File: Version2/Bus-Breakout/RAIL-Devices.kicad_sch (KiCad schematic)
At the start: 32 parts, among them J2 Conn_01x30_Pin, J5 Conn_02x30_Odd_Even, P1 Jumper4x1, P10 Jumper4x1, P11 Jumper4x1, P12 Jumper4x1, P13 Jumper4x1, P14 Jumper4x1, P15 Jumper4x1, P16 Jumper4x1, P17 Jumper4x1, P18 Jumper4x1, P19 Jumper4x1, P2 Jumper4x1, P20 Jumper4x1, P21 Jumper4x1, P22 Jumper4x1, P23 Jumper4x1, P24 Jumper4x1, P25 Jumper4x1, P26 Jumper4x1, P27 Jumper4x1, P28 Jumper4x1, P29 Jumper4x1, P3 Jumper4x1, P30 Jumper4x1, P4 Jumper4x1, P5 Jumper4x1, P6 Jumper4x1, P7 Jumper4x1, P8 Jumper4x1, P9 Jumper4x1

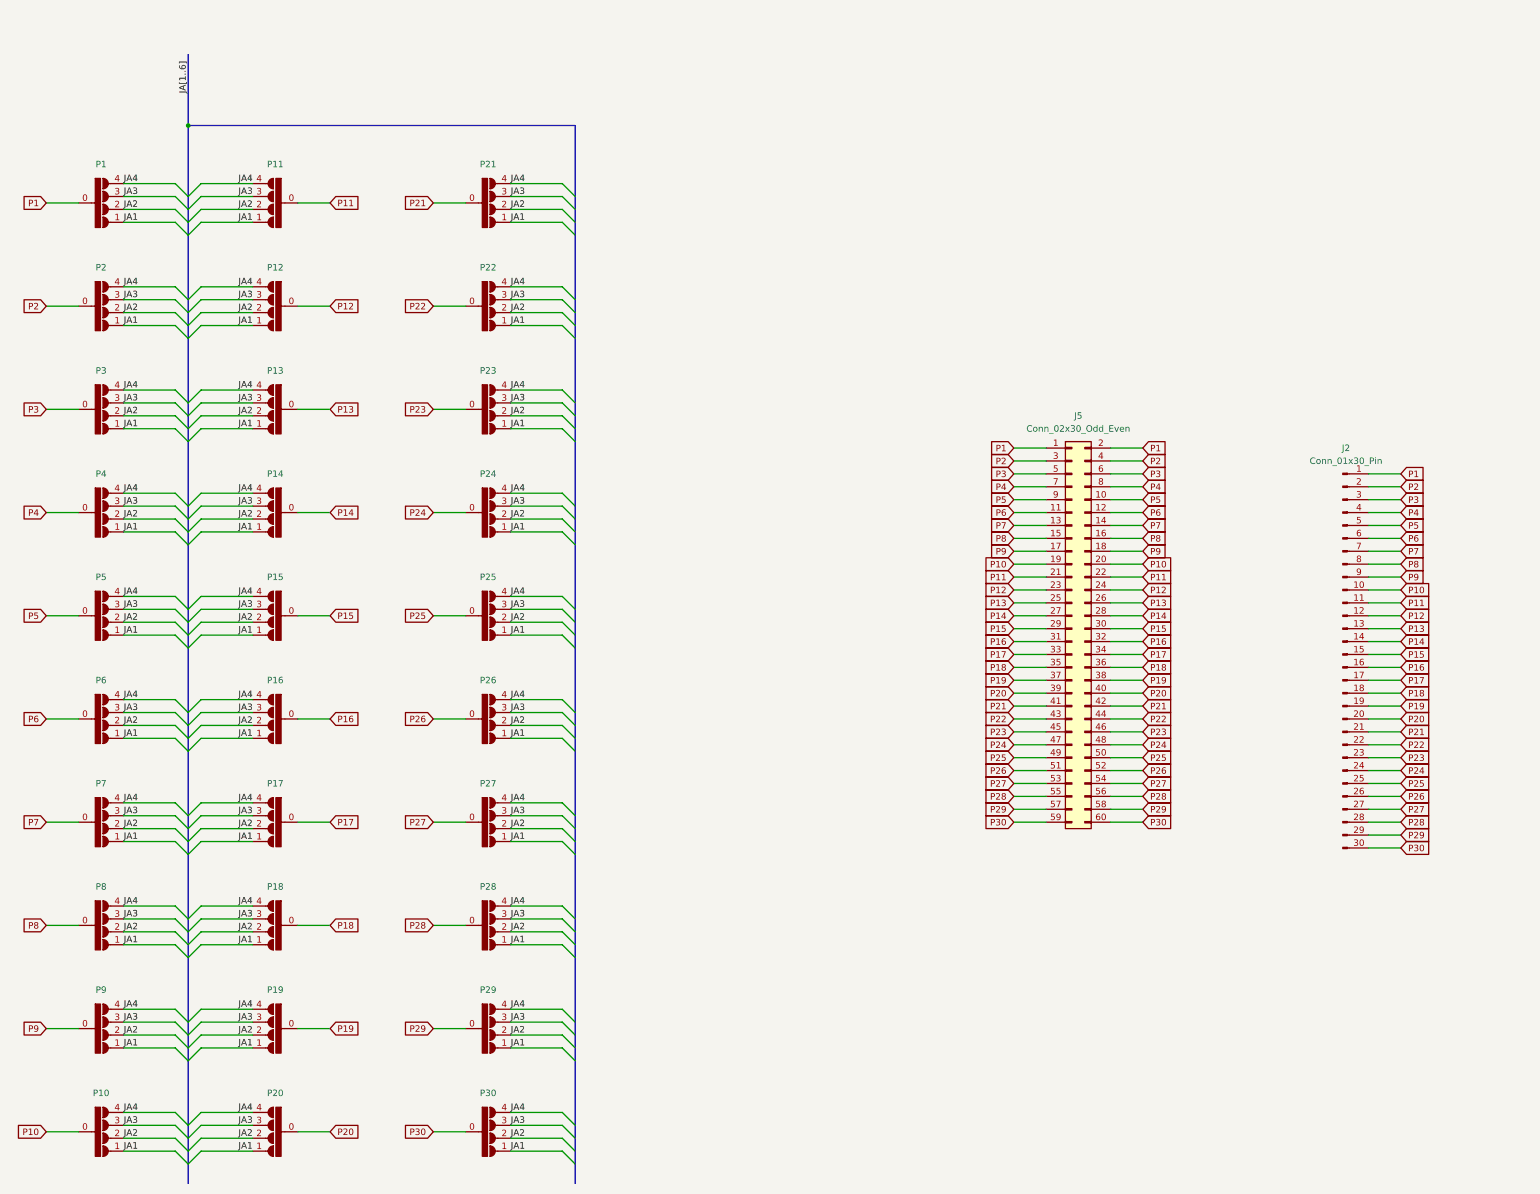
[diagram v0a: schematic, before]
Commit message: updates.
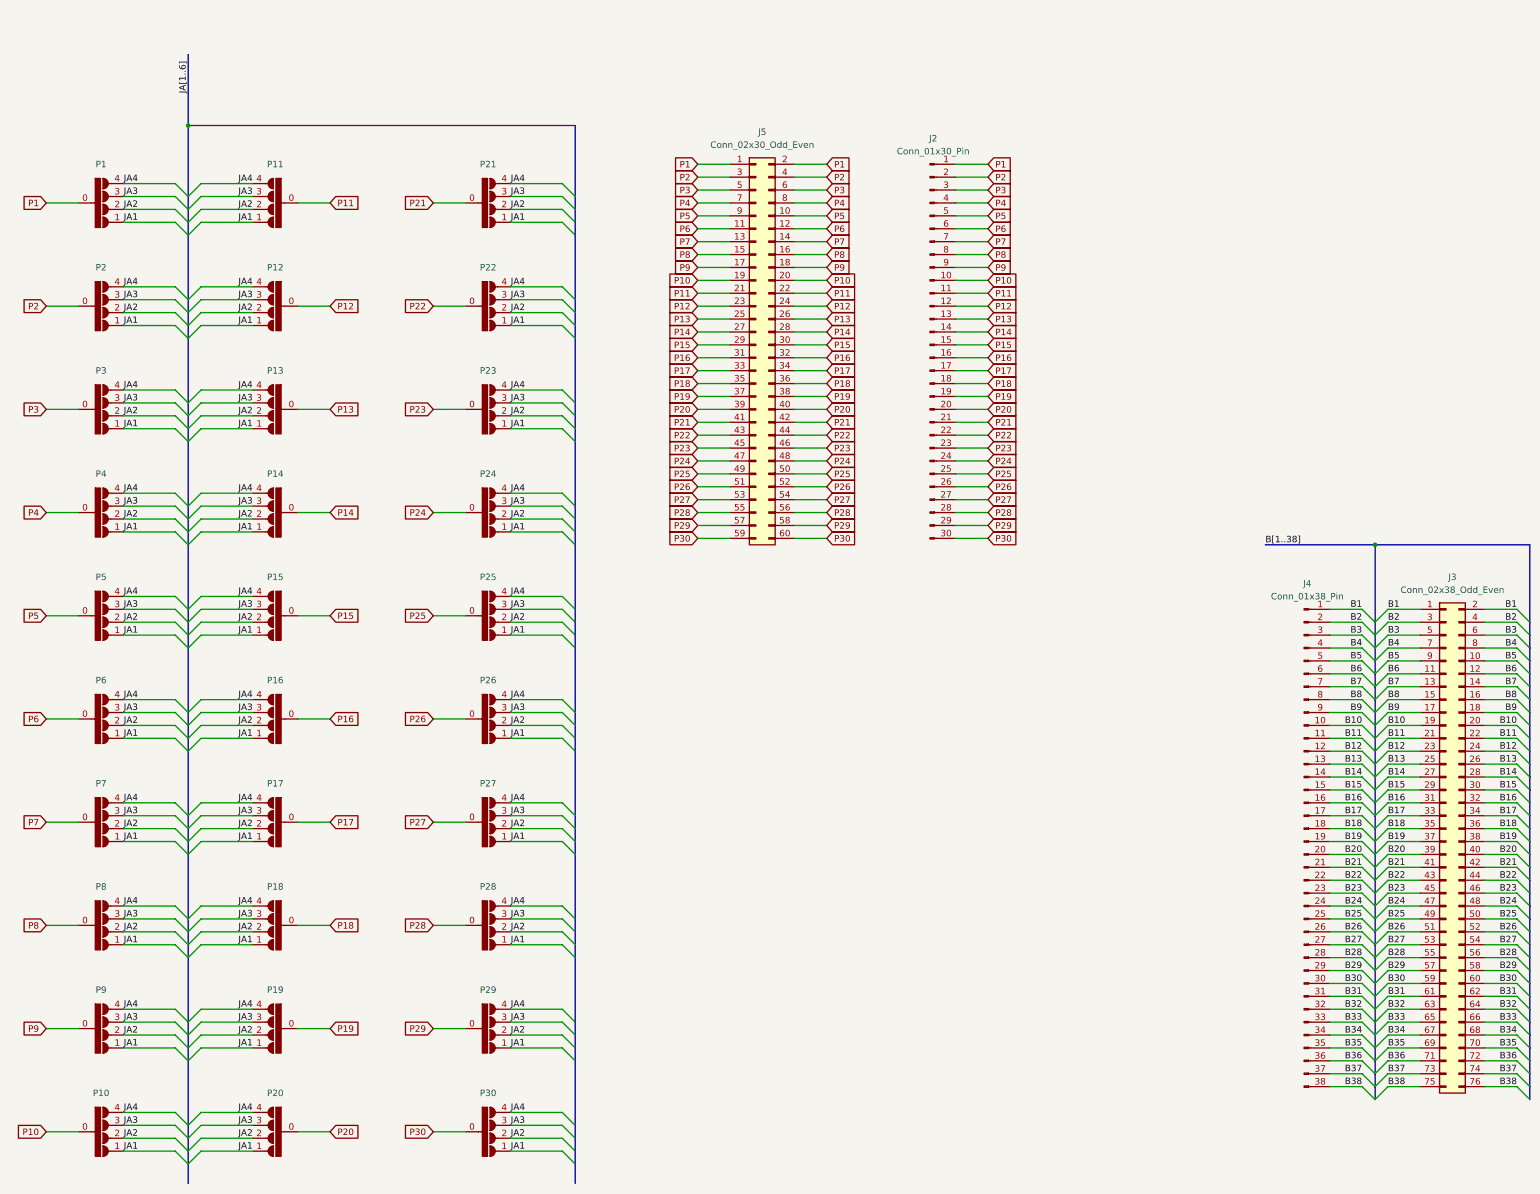
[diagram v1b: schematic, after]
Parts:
- added J3: Conn_02x38_Odd_Even, Connector_PinSocket_2.54mm:PinSocket_2x38_P2.54mm_Vertical, symbol Connector_Generic:Conn_02x38_Odd_Even
- added J4: Conn_01x38_Pin, Connector_PinSocket_2.54mm:PinSocket_1x38_P2.54mm_Vertical, symbol Connector:Conn_01x38_Pin
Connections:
- new net B1: J3.1 (Pin_1), J3.2 (Pin_2), J4.1 (Pin_1)
- new net B10: J3.19 (Pin_19), J3.20 (Pin_20), J4.10 (Pin_10)
- new net B11: J3.21 (Pin_21), J3.22 (Pin_22), J4.11 (Pin_11)
- new net B12: J3.23 (Pin_23), J3.24 (Pin_24), J4.12 (Pin_12)
- new net B13: J3.25 (Pin_25), J3.26 (Pin_26), J4.13 (Pin_13)
- new net B14: J3.27 (Pin_27), J3.28 (Pin_28), J4.14 (Pin_14)
- new net B15: J3.29 (Pin_29), J3.30 (Pin_30), J4.15 (Pin_15)
- new net B16: J3.31 (Pin_31), J3.32 (Pin_32), J4.16 (Pin_16)
- new net B17: J3.33 (Pin_33), J3.34 (Pin_34), J4.17 (Pin_17)
- new net B18: J3.35 (Pin_35), J3.36 (Pin_36), J4.18 (Pin_18)
- new net B19: J3.37 (Pin_37), J3.38 (Pin_38), J4.19 (Pin_19)
- new net B2: J3.3 (Pin_3), J3.4 (Pin_4), J4.2 (Pin_2)
- new net B20: J3.39 (Pin_39), J3.40 (Pin_40), J4.20 (Pin_20)
- new net B21: J3.41 (Pin_41), J3.42 (Pin_42), J4.21 (Pin_21)
- new net B22: J3.43 (Pin_43), J3.44 (Pin_44), J4.22 (Pin_22)
- new net B23: J3.45 (Pin_45), J3.46 (Pin_46), J4.23 (Pin_23)
- new net B24: J3.47 (Pin_47), J3.48 (Pin_48), J4.24 (Pin_24)
- new net B25: J3.49 (Pin_49), J3.50 (Pin_50), J4.25 (Pin_25)
- new net B26: J3.51 (Pin_51), J3.52 (Pin_52), J4.26 (Pin_26)
- new net B27: J3.53 (Pin_53), J3.54 (Pin_54), J4.27 (Pin_27)
- new net B28: J3.55 (Pin_55), J3.56 (Pin_56), J4.28 (Pin_28)
- new net B29: J3.57 (Pin_57), J3.58 (Pin_58), J4.29 (Pin_29)
- new net B3: J3.5 (Pin_5), J3.6 (Pin_6), J4.3 (Pin_3)
- new net B30: J3.59 (Pin_59), J3.60 (Pin_60), J4.30 (Pin_30)
- new net B31: J3.61 (Pin_61), J3.62 (Pin_62), J4.31 (Pin_31)
- new net B32: J3.63 (Pin_63), J3.64 (Pin_64), J4.32 (Pin_32)
- new net B33: J3.65 (Pin_65), J3.66 (Pin_66), J4.33 (Pin_33)
- new net B34: J3.67 (Pin_67), J3.68 (Pin_68), J4.34 (Pin_34)
- new net B35: J3.69 (Pin_69), J3.70 (Pin_70), J4.35 (Pin_35)
- new net B36: J3.71 (Pin_71), J3.72 (Pin_72), J4.36 (Pin_36)
- new net B37: J3.73 (Pin_73), J3.74 (Pin_74), J4.37 (Pin_37)
- new net B38: J3.75 (Pin_75), J3.76 (Pin_76), J4.38 (Pin_38)
- new net B4: J3.7 (Pin_7), J3.8 (Pin_8), J4.4 (Pin_4)
- new net B5: J3.10 (Pin_10), J3.9 (Pin_9), J4.5 (Pin_5)
- new net B6: J3.11 (Pin_11), J3.12 (Pin_12), J4.6 (Pin_6)
- new net B7: J3.13 (Pin_13), J3.14 (Pin_14), J4.7 (Pin_7)
- new net B8: J3.15 (Pin_15), J3.16 (Pin_16), J4.8 (Pin_8)
- new net B9: J3.17 (Pin_17), J3.18 (Pin_18), J4.9 (Pin_9)
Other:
- moved on the sheet: J2, J5

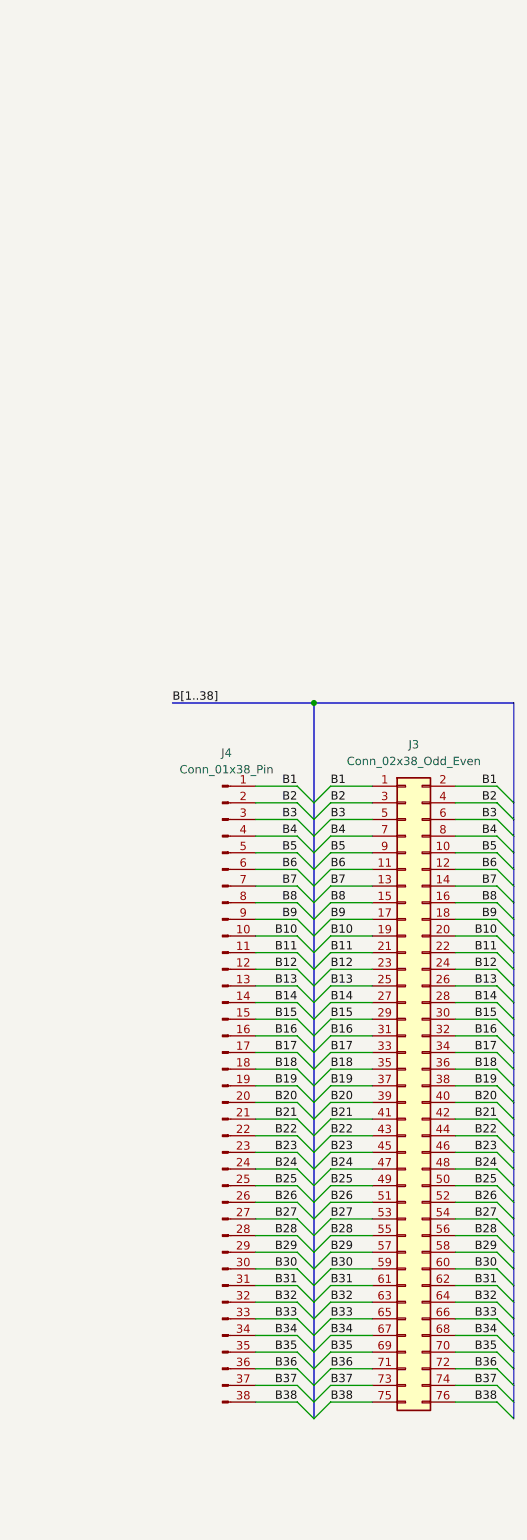
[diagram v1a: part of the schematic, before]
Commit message: update.
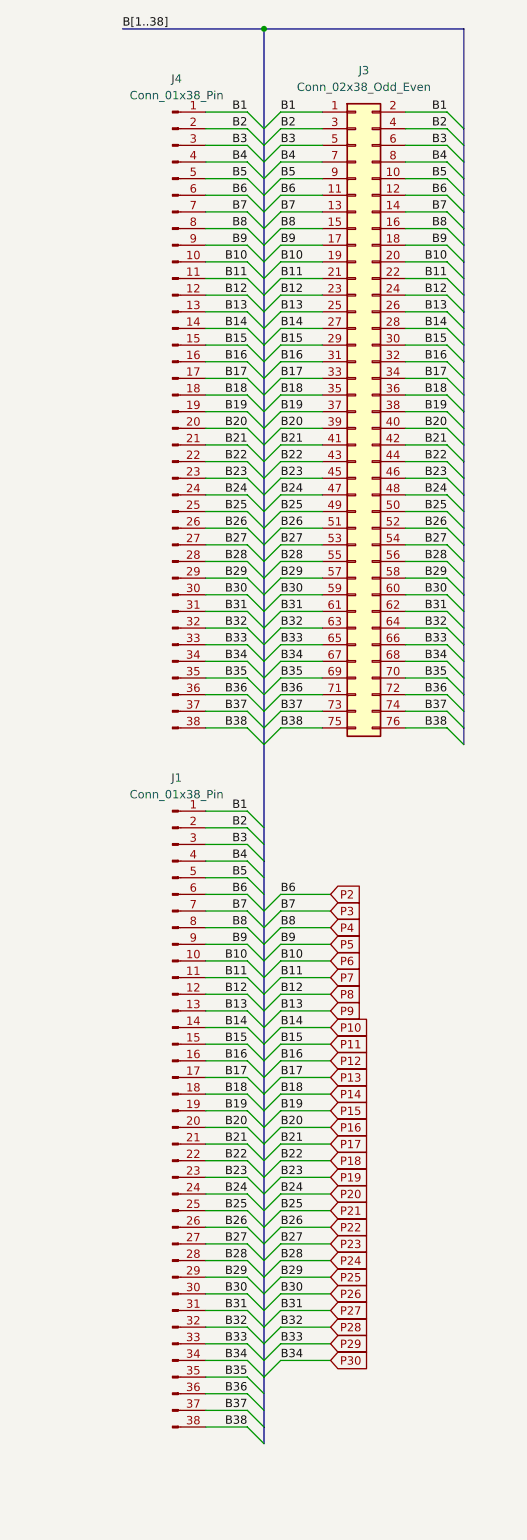
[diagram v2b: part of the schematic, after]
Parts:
- added J1: Conn_01x38_Pin, Connector_PinSocket_2.54mm:PinSocket_1x38_P2.54mm_Vertical, symbol Connector:Conn_01x38_Pin
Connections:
- net B10 is gone; now on net P6: J3.19 (Pin_19), J3.20 (Pin_20), J4.10 (Pin_10)
- net B11 is gone; now on net P7: J3.21 (Pin_21), J3.22 (Pin_22), J4.11 (Pin_11)
- net B12 is gone; now on net P8: J3.23 (Pin_23), J3.24 (Pin_24), J4.12 (Pin_12)
- net B13 is gone; now on net P9: J3.25 (Pin_25), J3.26 (Pin_26), J4.13 (Pin_13)
- net B14 is gone; now on net P10: J3.27 (Pin_27), J3.28 (Pin_28), J4.14 (Pin_14)
- net B15 is gone; now on net P11: J3.29 (Pin_29), J3.30 (Pin_30), J4.15 (Pin_15)
- net B16 is gone; now on net P12: J3.31 (Pin_31), J3.32 (Pin_32), J4.16 (Pin_16)
- net B17 is gone; now on net P13: J3.33 (Pin_33), J3.34 (Pin_34), J4.17 (Pin_17)
- net B18 is gone; now on net P14: J3.35 (Pin_35), J3.36 (Pin_36), J4.18 (Pin_18)
- net B19 is gone; now on net P15: J3.37 (Pin_37), J3.38 (Pin_38), J4.19 (Pin_19)
- net B20 is gone; now on net P16: J3.39 (Pin_39), J3.40 (Pin_40), J4.20 (Pin_20)
- net B21 is gone; now on net P17: J3.41 (Pin_41), J3.42 (Pin_42), J4.21 (Pin_21)
- net B22 is gone; now on net P18: J3.43 (Pin_43), J3.44 (Pin_44), J4.22 (Pin_22)
- net B23 is gone; now on net P19: J3.45 (Pin_45), J3.46 (Pin_46), J4.23 (Pin_23)
- net B24 is gone; now on net P20: J3.47 (Pin_47), J3.48 (Pin_48), J4.24 (Pin_24)
- net B25 is gone; now on net P21: J3.49 (Pin_49), J3.50 (Pin_50), J4.25 (Pin_25)
- net B26 is gone; now on net P22: J3.51 (Pin_51), J3.52 (Pin_52), J4.26 (Pin_26)
- net B27 is gone; now on net P23: J3.53 (Pin_53), J3.54 (Pin_54), J4.27 (Pin_27)
- net B28 is gone; now on net P24: J3.55 (Pin_55), J3.56 (Pin_56), J4.28 (Pin_28)
- net B29 is gone; now on net P25: J3.57 (Pin_57), J3.58 (Pin_58), J4.29 (Pin_29)
- net B30 is gone; now on net P26: J3.59 (Pin_59), J3.60 (Pin_60), J4.30 (Pin_30)
- net B31 is gone; now on net P27: J3.61 (Pin_61), J3.62 (Pin_62), J4.31 (Pin_31)
- net B32 is gone; now on net P28: J3.63 (Pin_63), J3.64 (Pin_64), J4.32 (Pin_32)
- net B33 is gone; now on net P29: J3.65 (Pin_65), J3.66 (Pin_66), J4.33 (Pin_33)
- net B34 is gone; now on net P30: J3.67 (Pin_67), J3.68 (Pin_68), J4.34 (Pin_34)
- net B6 is gone; now on net P2: J3.11 (Pin_11), J3.12 (Pin_12), J4.6 (Pin_6)
- net B7 is gone; now on net P3: J3.13 (Pin_13), J3.14 (Pin_14), J4.7 (Pin_7)
- net B8 is gone; now on net P4: J3.15 (Pin_15), J3.16 (Pin_16), J4.8 (Pin_8)
- net B9 is gone; now on net P5: J3.17 (Pin_17), J3.18 (Pin_18), J4.9 (Pin_9)
- net B1: now also J1.1 (Pin_1)
- net B2: now also J1.2 (Pin_2)
- net B3: now also J1.3 (Pin_3)
- net B35: now also J1.35 (Pin_35)
- net B36: now also J1.36 (Pin_36)
- net B37: now also J1.37 (Pin_37)
- net B38: now also J1.38 (Pin_38)
- net B4: now also J1.4 (Pin_4)
- net B5: now also J1.5 (Pin_5)
- net P10: now also J1.14 (Pin_14)
- net P11: now also J1.15 (Pin_15)
- net P12: now also J1.16 (Pin_16)
- net P13: now also J1.17 (Pin_17)
- net P14: now also J1.18 (Pin_18)
- net P15: now also J1.19 (Pin_19)
- net P16: now also J1.20 (Pin_20)
- net P17: now also J1.21 (Pin_21)
- net P18: now also J1.22 (Pin_22)
- net P19: now also J1.23 (Pin_23)
- net P2: now also J1.6 (Pin_6)
- net P20: now also J1.24 (Pin_24)
- net P21: now also J1.25 (Pin_25)
- net P22: now also J1.26 (Pin_26)
- net P23: now also J1.27 (Pin_27)
- net P24: now also J1.28 (Pin_28)
- net P25: now also J1.29 (Pin_29)
- net P26: now also J1.30 (Pin_30)
- net P27: now also J1.31 (Pin_31)
- net P28: now also J1.32 (Pin_32)
- net P29: now also J1.33 (Pin_33)
- net P3: now also J1.7 (Pin_7)
- net P30: now also J1.34 (Pin_34)
- net P4: now also J1.8 (Pin_8)
- net P5: now also J1.9 (Pin_9)
- net P6: now also J1.10 (Pin_10)
- net P7: now also J1.11 (Pin_11)
- net P8: now also J1.12 (Pin_12)
- net P9: now also J1.13 (Pin_13)
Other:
- moved on the sheet: J3, J4
